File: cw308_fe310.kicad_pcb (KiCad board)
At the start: 2 copper layers, 56 x 67 mm, 51 parts, among them J1 CW308T_CONNBOARD, J2 Conn_02x03_Odd_Even, J4 Conn_02x05_Odd_Even, J5 10118192-0001LF, U1 IS25LP128, U2 SN74LVC1G07DBVR, U3 SN74LVC1G07DBVR, U4 FE310-G000, U5 FT2232HL-REEL, Y1 12MHz

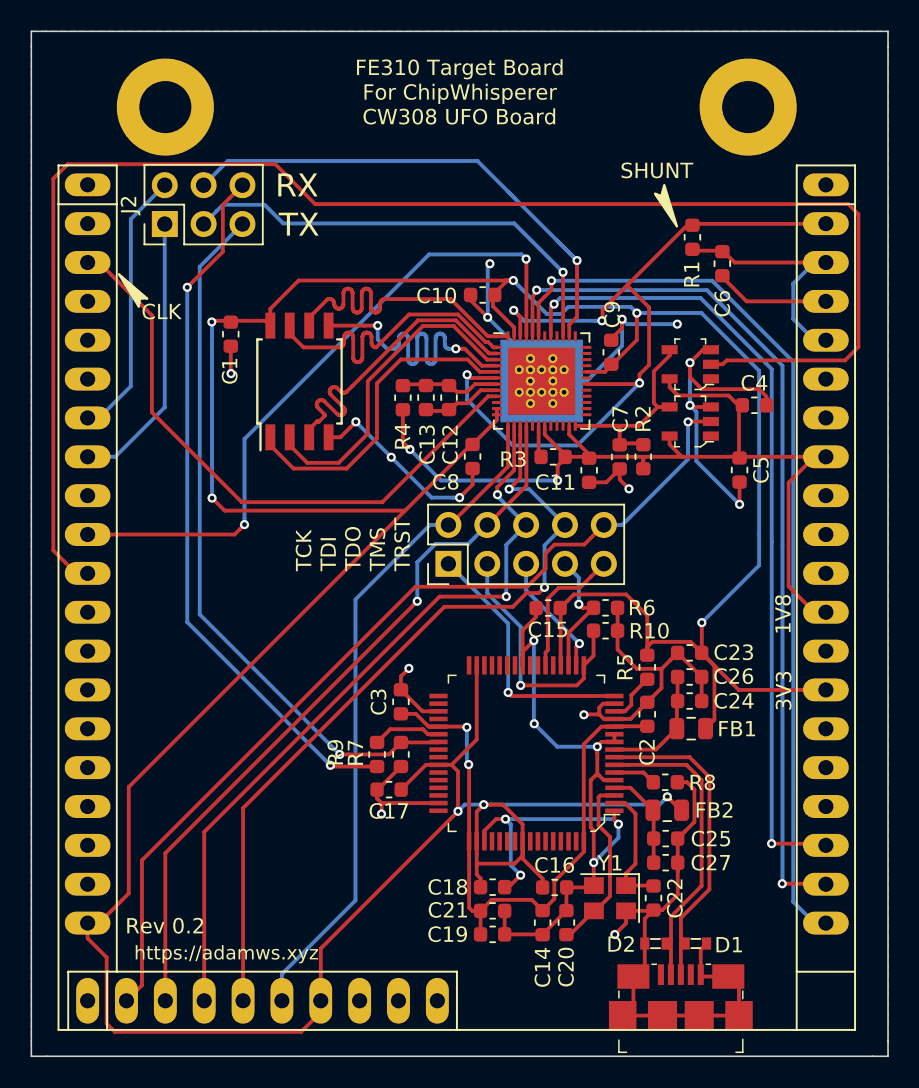
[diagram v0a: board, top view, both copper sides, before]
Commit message: order made
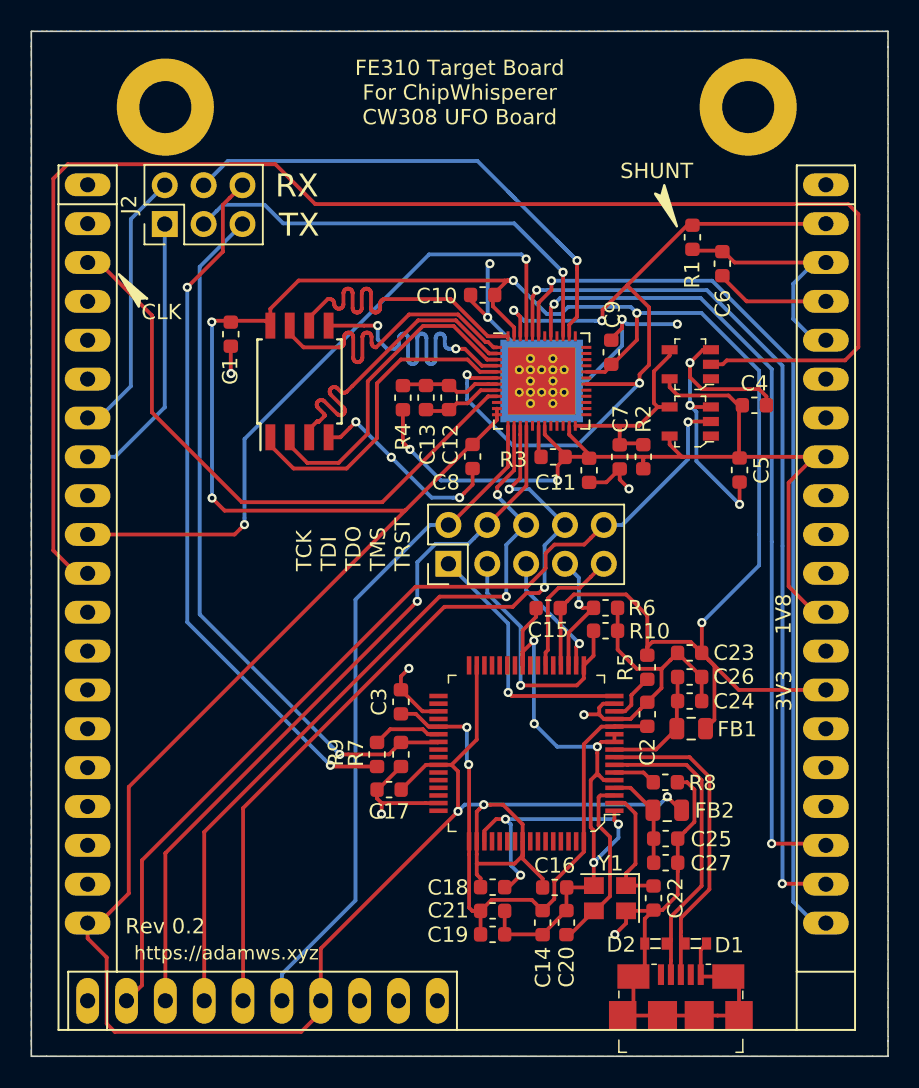
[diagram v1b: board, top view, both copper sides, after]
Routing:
- added copper zone on B.Cu, net (none)
- added copper zone on F.Cu, net GND
- removed copper zone on B.Cu, net GND
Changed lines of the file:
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@@
   (page A4)
   (layers
-    (0 F.Cu signal hide)
-    (31 B.Cu signal hide)
+    (0 F.Cu signal)
+    (31 B.Cu signal)
     (32 B.Adhes user hide)
     (33 F.Adhes user hide)
@@
     (visible_elements FFFFFFFF)
     (pcbplotparams
-      (layerselection 0x010fc_ffffffff)
+      (layerselection 0x010f0_ffffffff)
       (usegerberextensions false)
-      (usegerberattributes false)
+      (usegerberattributes true)
       (usegerberadvancedattributes false)
       (creategerberjobfile false)
       (excludeedgelayer true)
-      (linewidth 0.100000)
+      (linewidth 0.150000)
       (plotframeref false)
       (viasonmask false)
@@
   (segment (start 151.76246 94.0816) (end 152.47112 93.37294) (width 0.25) (layer F.Cu) (net 113))
   (segment (start 153.85542 93.37294) (end 154.572601 92.655759) (width 0.25) (layer F.Cu) (net 113))
-  (zone (net 1) (net_name GND) (layer B.Cu) (hatch edge 0.508)
+  (zone (net 1) (net_name GND) (layer F.Cu) (hatch edge 0.508)
     (connect_pads (clearance 0.508))
     (min_thickness 0.254)
@@
       )
     )
+  )
+  (zone (net 0) (net_name "") (layer B.Cu) (hatch edge 0.508)
+    (connect_pads (clearance 0.508))
+    (min_thickness 0.254)
+    (fill yes (arc_segments 16) (thermal_gap 0.508) (thermal_bridge_width 0.508))
+    (polygon
+      (pts
+        (xy 117.9957 56.9976) (xy 117.9957 124.0028) (xy 174.0027 124.0028) (xy 174.0027 56.9976)
+      )
+    )
